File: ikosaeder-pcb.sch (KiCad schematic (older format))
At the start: 5 parts, among them J1 Conn_01x03_Female, J2 Conn_01x03_Female, J3 Conn_01x03_Female, J4 Conn_01x03_Female, J5 Conn_01x03_Female

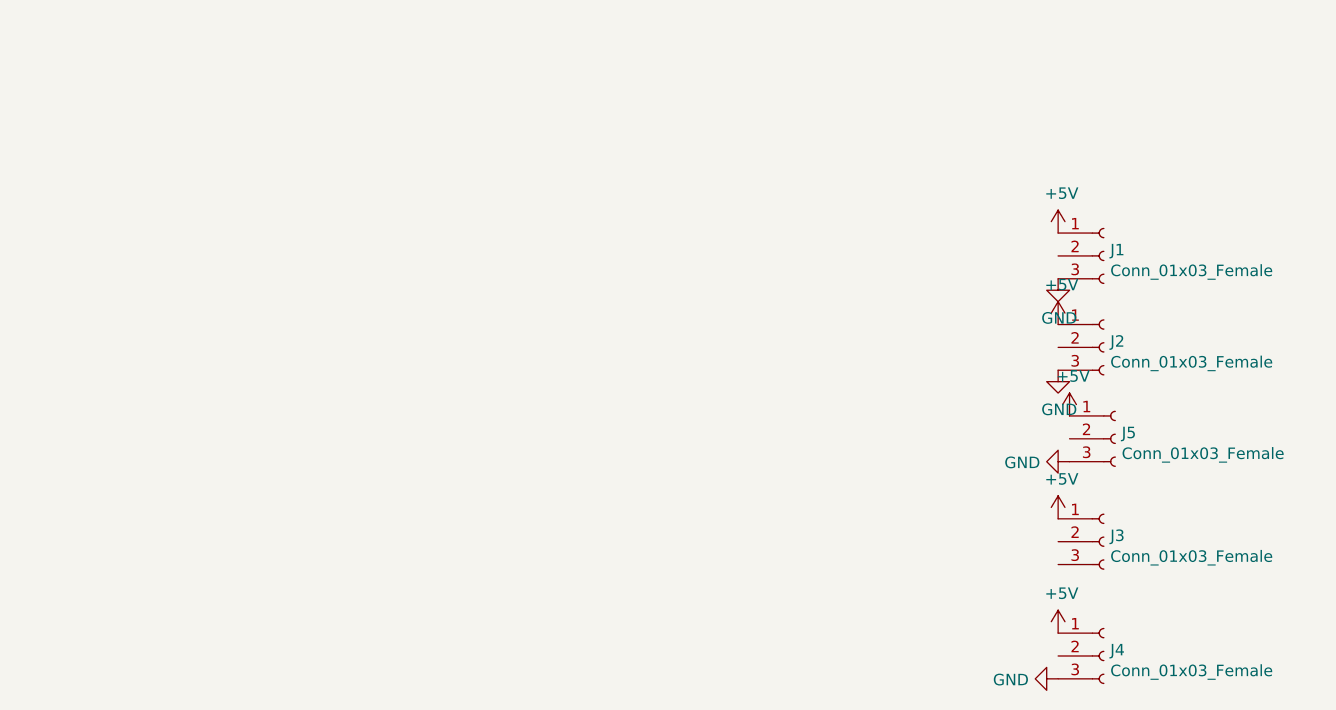
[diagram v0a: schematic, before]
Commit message: Make the first pcb board which has the label A
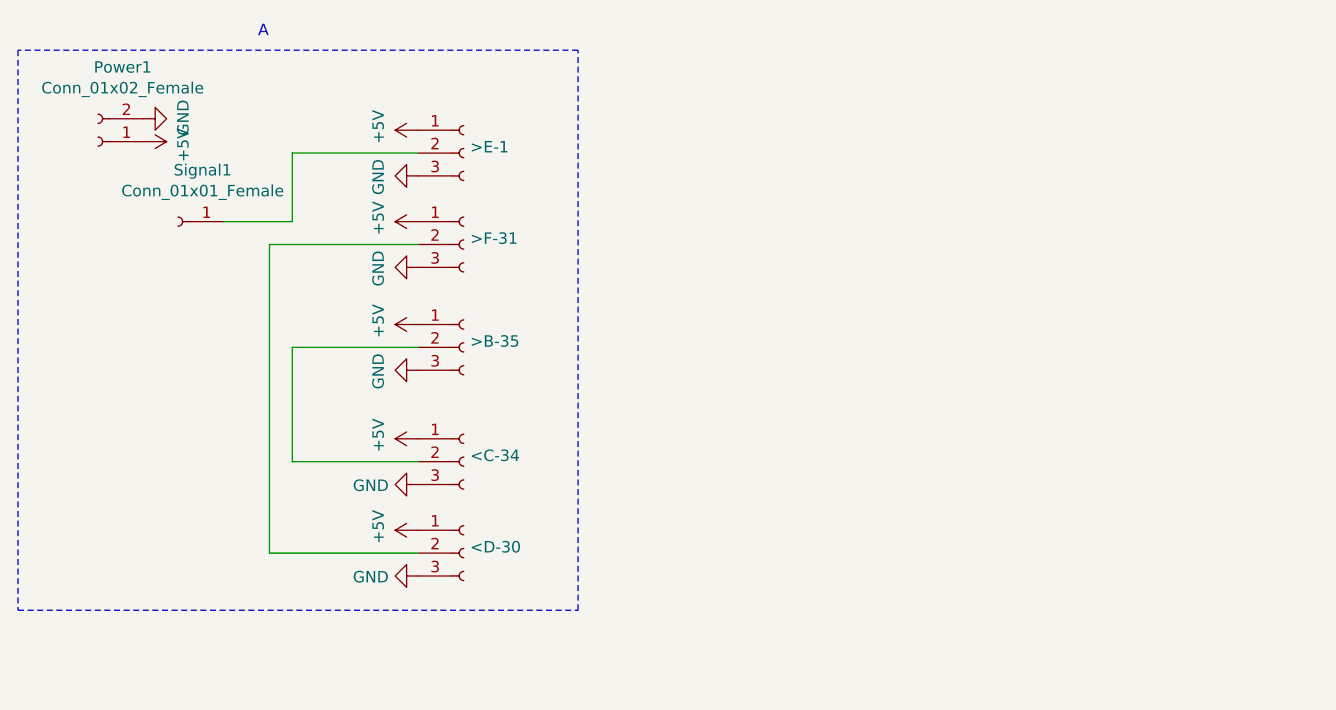
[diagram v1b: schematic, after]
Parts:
- added Power1: Conn_01x02_Female, Connector_PinHeader_2.54mm:PinHeader_1x02_P2.54mm_Vertical, symbol Connector:Conn_01x02_Female
- added Signal1: Conn_01x01_Female, Connector_PinHeader_2.54mm:PinHeader_1x01_P2.54mm_Vertical, symbol Connector:Conn_01x01_Female
- renumbered J4 to <C-34, J5 to <D-30, J3 to >B-35, J1 to >E-1, J2 to >F-31
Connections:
- net +5V: now also Power1.1 (Pin_1)
- net GND: now also >B-35.3 (Pin_3), Power1.2 (Pin_2)
- net at >E-1.2 (Pin_2): now also Signal1.1 (Pin_1)
- net at >F-31.2 (Pin_2): now also <D-30.2 (Pin_2)
- net at >B-35.2 (Pin_2): now also <C-34.2 (Pin_2)
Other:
- note added: "A"
- moved on the sheet: <C-34, <D-30, >B-35, >E-1, >F-31
